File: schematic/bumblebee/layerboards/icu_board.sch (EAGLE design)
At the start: 1 part

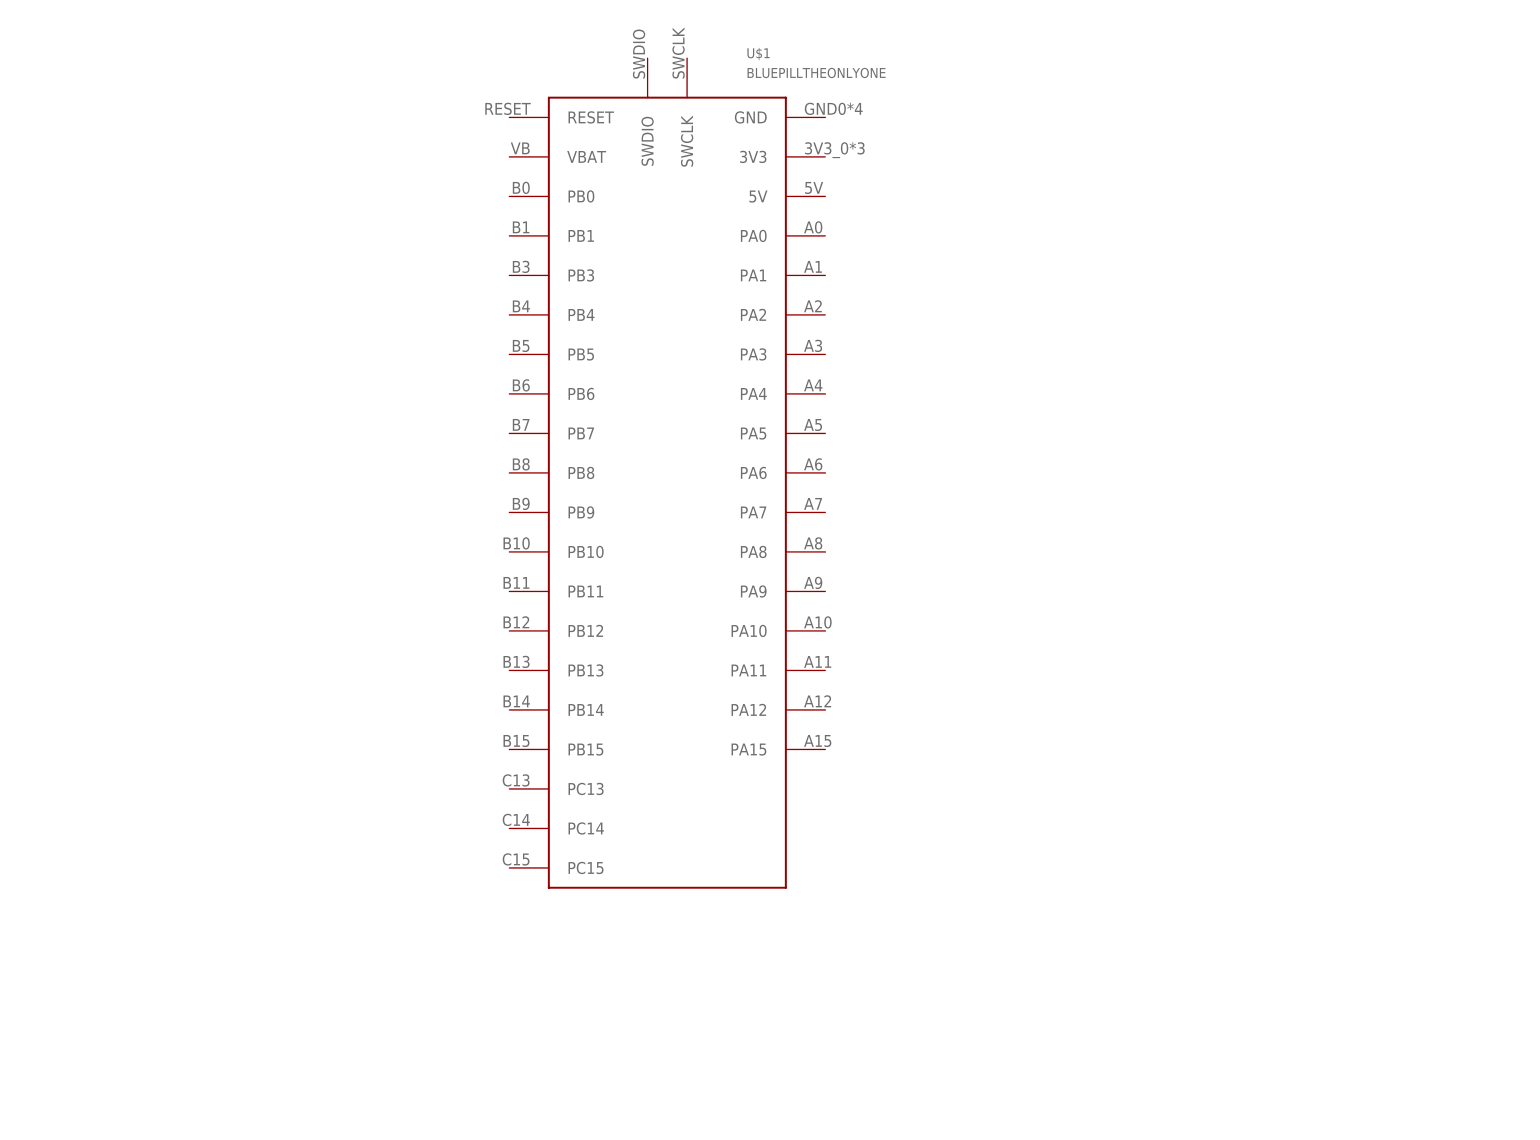
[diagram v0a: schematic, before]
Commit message: RC платок аппарата
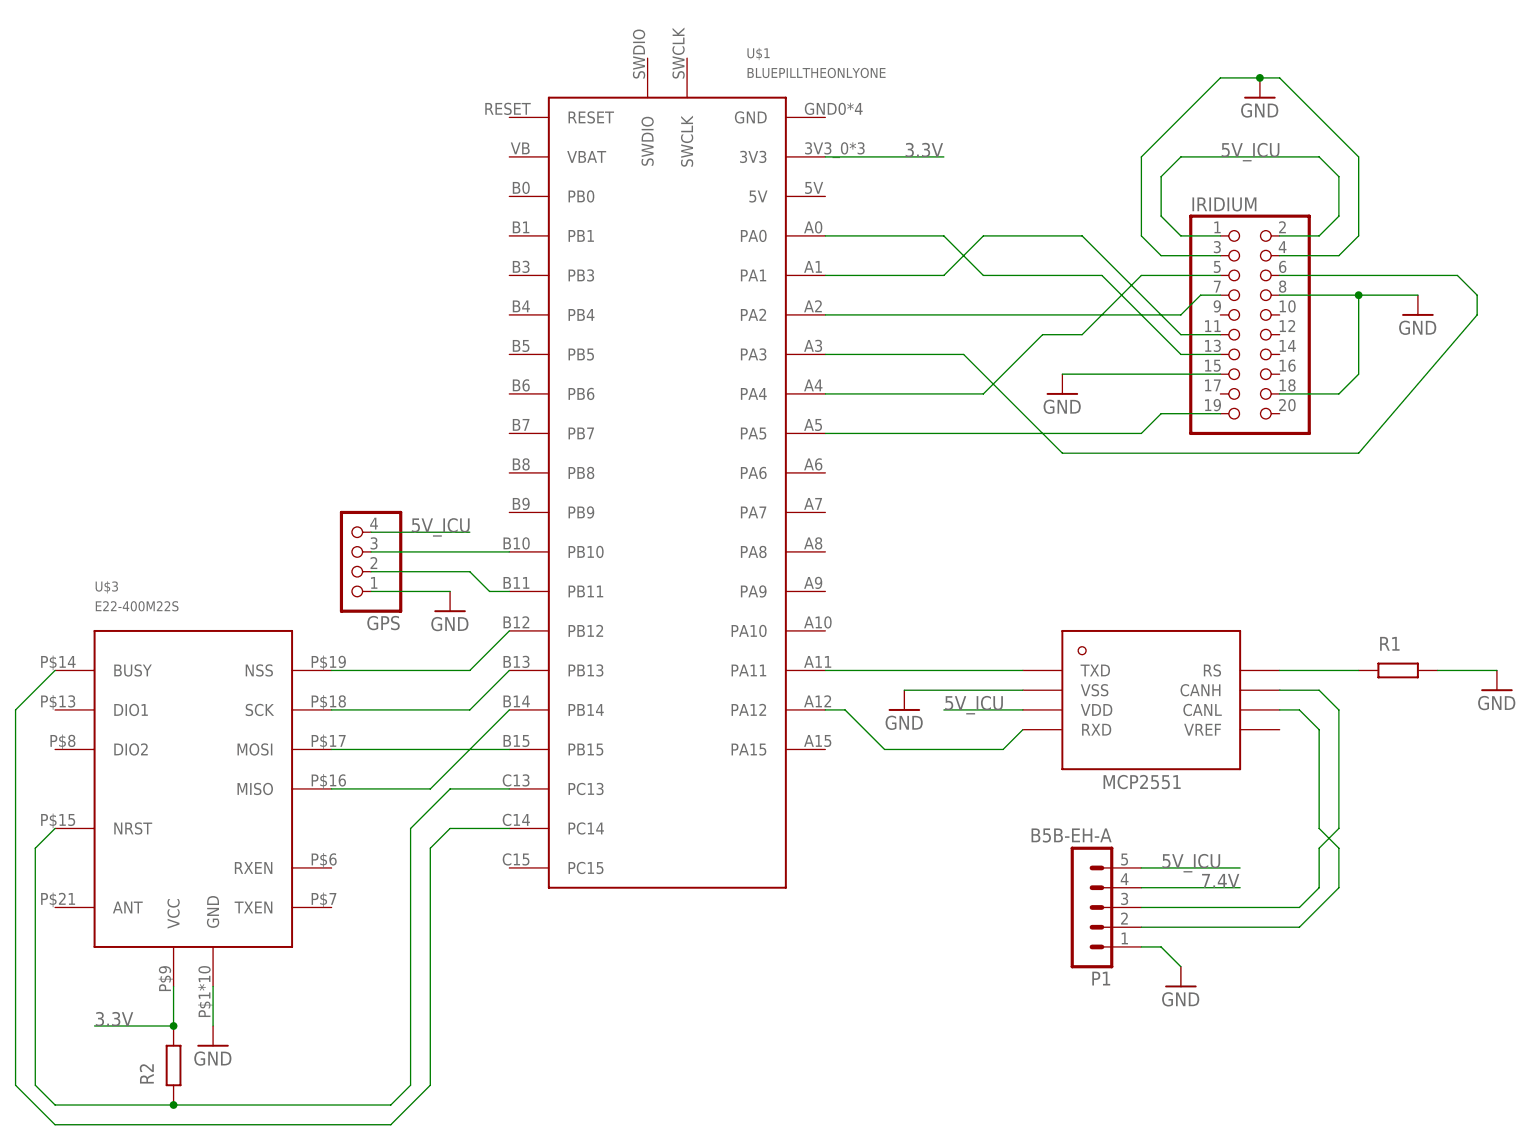
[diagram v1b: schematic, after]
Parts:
- added GPS: (no value), pinhead:PINHD-1X4
- added IRIDIUM: (no value), pinhead:PINHD-2X10
- added P1: B5B-EH-A, con-jst-eh:B5B-EH-A
- added R1, R2: (no value), ngspice-simulation:R
- added U$2: MCP2551, MCP2551:MCP2551
- added U$3: E22-400M22S, ebyte-radio:E22-400M22S
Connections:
- new net 3.3V: R2.2, U$1.3V3, U$3.VCC
- new net 5V_ICU: GPS.4, IRIDIUM.1, IRIDIUM.2, P1.5, U$2.VDD
- new net 7.4V: P1.4
- new net GND: GPS.1, IRIDIUM.15, IRIDIUM.18, IRIDIUM.3, IRIDIUM.4, IRIDIUM.8, P1.1, R1.2, U$2.VSS, U$3.GND
- new net N$1: IRIDIUM.5, U$1.PA4
- new net N$10: U$1.PA12, U$2.RXD
- new net N$11: R1.1, U$2.RS
- new net N$12: P1.3, U$2.CANH
- new net N$13: P1.2, U$2.CANL
- new net N$14: U$1.PB12, U$3.NSS
- new net N$15: U$1.PB13, U$3.SCK
- new net N$16: U$1.PB15, U$3.MOSI
- new net N$17: U$1.PB14, U$3.MISO
- new net N$18: R2.1, U$1.PC13, U$3.NRST
- new net N$19: U$1.PC14, U$3.BUSY
- new net N$2: GPS.3, U$1.PB10
- new net N$3: IRIDIUM.11, U$1.PA1
- new net N$4: IRIDIUM.13, U$1.PA0
- new net N$5: IRIDIUM.7, U$1.PA2
- new net N$6: IRIDIUM.6, U$1.PA3
- new net N$7: IRIDIUM.19, U$1.PA5
- new net N$8: GPS.2, U$1.PB11
- new net N$9: U$1.PA11, U$2.TXD
